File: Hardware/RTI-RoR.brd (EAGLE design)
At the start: 80 x 71.1 mm, 49 parts, among them IC1 24AA128ST, IC3 FT232RL, IC5 74LVC245, IC6 74ABT245, X13 PN61729-S

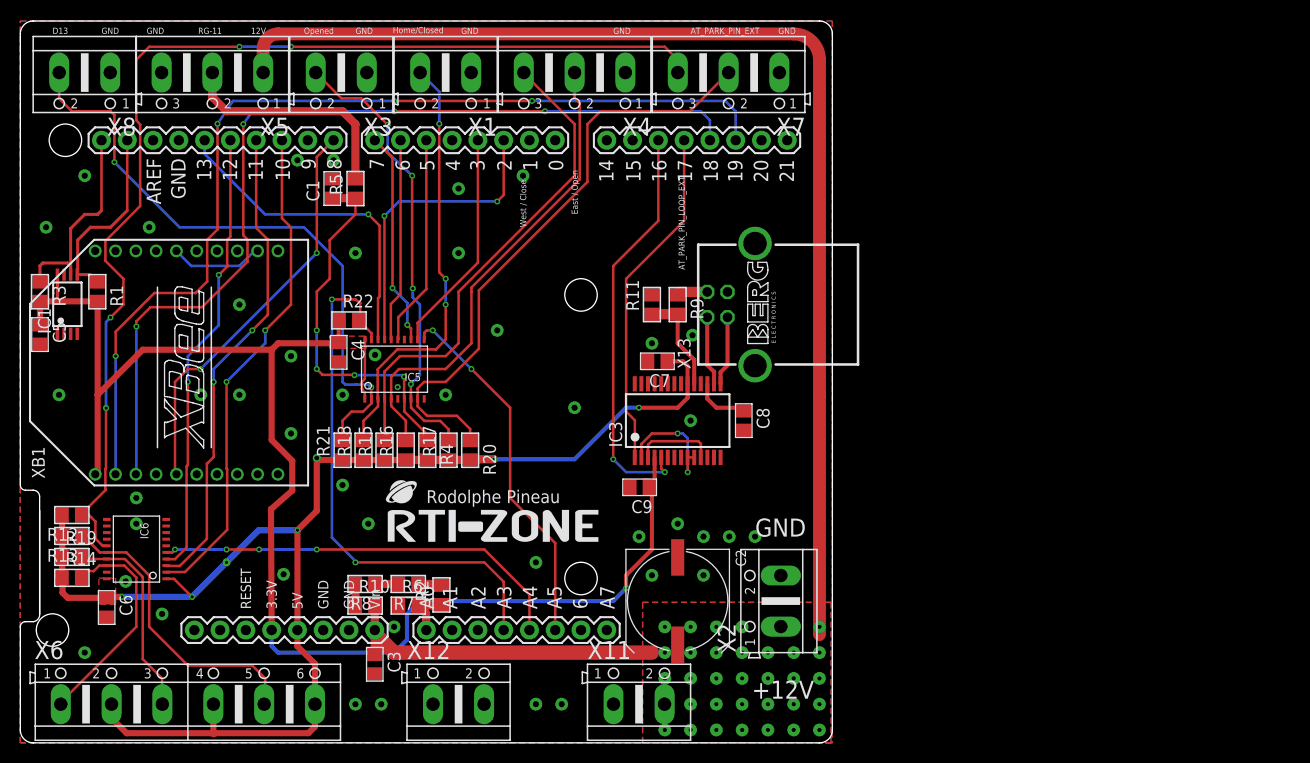
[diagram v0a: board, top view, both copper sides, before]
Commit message: Re-base the code with the dome code
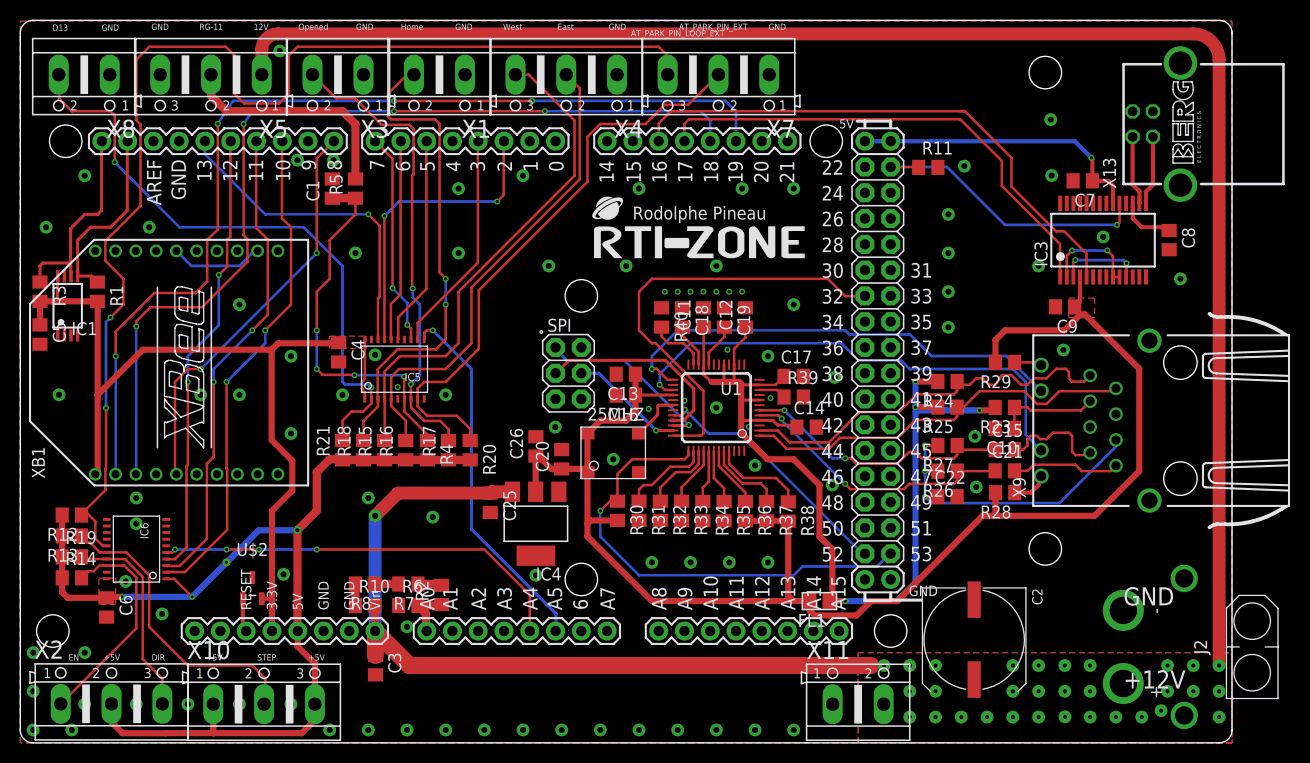
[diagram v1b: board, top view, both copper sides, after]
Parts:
- removed PCB1: ARDUINO_DUE_SHIELD_SHORT, arduino_shield:ARDUINO_DUE_SHIELD_SHORT
- removed R22, R9: 4.7K, rti:R0805
- removed X12: (no value), con-ptr500:AK500/2
- removed X6: (no value), con-ptr500:AK500/6
- added 25MHZ: CB3LV-OSCILATOR, rti:SMD-7050_4P
- added C10: 22nF, rcl:C0805
- added C11, C12, C14, C16, C17, C20: 100nF, rcl:C0805
- added C13, C18, C22: 10nF, rcl:C0805
- added C15, C21: 6.8nF, rcl:C0805
- added C19: 4.7uF, rcl:C0805
- added C25, C26: 10uF, rcl:C0805
- added FL1: BLM21AG121SN1D, BLM21AG121SN1D:L0805
- added IC4: REG1117, burr-brown:SOT223
- added J2: XT60PW-M, samacsys:XT60PWM
- added R23: 10 1%, rcl:R0805
- added R24, R25, R26, R27: 49.9 1%, rcl:R0805
- added R28, R29: 330, rcl:R0805
- added R30, R31, R32, R33, R34, R35, R36, R37, R38, R40: 4.7K, rcl:R0805
- added R39: 12.4K 1%, rcl:R0805
- added U$1: ARDUINO_DUE_SHIELD_FULL, arduino_shield:ARDUINO_DUE_SHIELD_FULL
- added U$2: MCP120T-270I_TT, MCP120T-270I_TT:SOT95P237X112-3N
- added U1: W5500, W5500:LQFP48
- added X10: (no value), rti:AK500/3
- added X9: J1011F21PNL, rti:J1011F21PNL
- C1, C3, C4, C5, C6, C7, C8, C9: device rti:C0805 -> rcl:C0805
- C2: device rti:UD-10X10_NICHICON -> rcl:UD-10X10_NICHICON
- IC1: device microchip:TSSOP8 -> rti:TSSOP8
- R1, R10, R11, R12, R13, R14, R15, R16, R17, R18, R19, R2, R20, R21, R3, R4, R5, R6, R7, R8: device rti:R0805 -> rcl:R0805
- X1, X11, X3, X8: device con-ptr500:AK500/2 -> rti:AK500/2
- X13: device con-berg:PN61729-S -> rti:PN61729-S
- X2: device con-ptr500:AK500/2 -> rti:AK500/3
- X4, X5, X7: device con-ptr500:AK500/3 -> rti:AK500/3
- XB1: device maxstream:XBEE -> rti:XBEE
- moved X2 66.7 mm to (8.99, 3.84), turned to 0 degrees
- moved IC3 45.5 mm to (106.7, 49.5)
- moved C7 45.5 mm to (104.7, 55.4)
- moved C8 45.5 mm to (113.2, 49.5)
- moved C9 45.5 mm to (102.9, 43.0)
- moved X13 45.5 mm to (114.3, 61.0)
- moved U$4 34.5 mm to (56.5, 47.8)
- moved R11 30.4 mm to (89.5, 56.7), turned to 0 degrees
- moved C2 29.5 mm to (94.0, 10.2)
- moved X11 21.6 mm to (82.5, 3.81)
- moved X7 1.02 mm to (68.8, 65.8)
- moved X4 0.85 mm to (53.8, 65.8)
- moved X1 0.64 mm to (41.3, 65.8)
- moved X3 0.38 mm to (31.3, 65.8)
- moved X5 0.24 mm to (18.8, 65.8)
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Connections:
- removed net BUF_EN: IC5.P$19, PCB1.A3, R22.2
- removed net N$1: IC3.19, R11.1, R9.2
- new net +3V3: 25MHZ.1, 25MHZ.4, C13.1, C16.1, C20.1, C26.1, C9.1, FL1.2, IC3.4, IC4.2, R28.2, R29.2, R30.2, R36.2, R37.2, R38.2, U1.28
- new net +5V: U$1.+5V@2
- new net ACT_LED: U1.27, X9.11
- new net AVDD: C11.1, C12.1, C14.1, C17.1, FL1.1, R23.2, R24.2, R25.2, U1.11, U1.15, U1.17, U1.21, U1.4, U1.8
- new net ETH_CS: U$1.52, U1.32
- new net ETH_RESET: R30.1, U$1.53, U1.37
- new net FTDI_RESET: IC3.19, R11.1, U$1.23
- new net INT_N: U$1.32, U1.36
- new net LINK_ACK: U1.25, X9.10
- new net N$10: R28.1, X9.12
- new net N$11: C15.2, X9.7
- new net N$12: C21.2, X9.8
- new net N$13: C10.1, R23.1, X9.3
- new net N$17: U1.26
- new net N$22: R31.1, U1.38
- new net N$23: R32.1, U1.39
- new net N$24: R33.1, U1.40
- new net N$25: R34.1, U1.41
- new net N$26: R35.1, U1.42
- new net N$27: R36.1, U1.43
- new net N$28: R37.1, U1.44
- new net N$29: R38.1, U1.45
- new net N$31: C19.2, U1.20
- new net N$32: U1.18
- new net N$33: C18.2, U1.22
- new net N$34: R39.1, U1.10
- new net N$35: R40.2, U1.23
- new net N$7: C22.1, R26.2, R27.2, X9.6
- new net N$8: R29.1, X9.9
- new net RESET: U$1.RESET, U$2.1
- new net RXN: C21.1, R26.1, U1.5
- new net RXP: C15.1, R27.1, U1.6
- new net SCLK: U$1.SCK, U1.33
- new net SDI: U$1.MISO, U1.34
- new net SDO: U$1.MOSI, U1.35
- new net TXN: R25.1, U1.1, X9.2
- new net TXP: R24.1, U1.2, X9.1
- new net XI: 25MHZ.3, U1.30
- new net XO: U1.31
- net +12V: now also C25.1, IC4.3, J2.2, U$1.VIN; no longer PCB1.VIN, X2.1
- net 3.3V: now also U$1.3.3V, U$2.2; no longer C9.1, IC3.4, PCB1.3.3V, R22.1
- net AT_PARK_PIN: now also U$1.A5; no longer PCB1.A5
- net AT_PARK_PIN_LOOP: now also U$1.A4; no longer PCB1.A4
- net BUTTON_EAST_OPEN: now also U$1.5; no longer PCB1.5
- net BUTTON_WEST_CLOSE: now also U$1.6; no longer PCB1.6
- net D13: now also U$1.13; no longer PCB1.13
- net GND: now also 25MHZ.2, C10.2, C11.2, C12.2, C13.2, C14.2, C16.2, C17.2, C18.1, C19.1, C20.2, C22.2, C25.2, C26.2, IC4.1, IC5.P$19, J2.1, R31.2, R32.2, R33.2, R34.2, R35.2, R39.2, R40.1, U$1.GND, U$1.GND., U$1.GND.., U$1.GND..., U$1.GND...., U$1.GND__, U$2.3, U1.14, U1.16, U1.19, U1.29, U1.3, U1.48, U1.9, X9.4, X9.5, X9.M1, X9.M2; no longer PCB1.GND, PCB1.GND., PCB1.GND.., X12.1, X12.2, X2.2
- net HOME_SHUTTER_CLOSED: now also U$1.2; no longer PCB1.2
- net M_DIR: now also U$1.11; no longer PCB1.11
- net M_DIR_5V: now also X2.3; no longer X6.3
- net M_EN: now also U$1.10; no longer PCB1.10
- net M_EN_5V: now also X2.1; no longer X6.1
- net M_STEP: now also U$1.12; no longer PCB1.12
- net M_STEP_5V: now also X10.2; no longer X6.5
- net RG-11: now also U$1.7; no longer PCB1.7
- net RX2: now also U$1.17; no longer PCB1.17
- net SCL: now also U$1.SCL1; no longer PCB1.SCL1
- net SDA: now also U$1.SDA1; no longer PCB1.SDA1
- net SHUTTER_OPENED: now also U$1.3; no longer PCB1.3
- net TX2: now also U$1.16; no longer PCB1.16
- net USB_VCC: no longer R9.1
- net VCC: now also U$1.+5V@1, U$1.+5V@3, U$1.+5V@4, X10.1, X10.3, X2.2; no longer PCB1.5V, X6.2, X6.4, X6.6
- net VPIN: now also U$1.A0; no longer PCB1.A0
- net XBEE_DIN: now also U$1.18; no longer PCB1.18
- net XBEE_DOUT: now also U$1.19; no longer PCB1.19
- net XBEE_RESET: now also U$1.8; no longer PCB1.8
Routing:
- net +3V3: track 0.00 -> 146.7 mm
- net AVDD: track 0.00 -> 96.8 mm, vias 0 -> 4
- net +12V: track 148.7 -> 239.2 mm
- net 3.3V: track 146.4 -> 90.1 mm, vias 1 -> 0
- net BUF_EN: track 54.1 -> 0.00 mm, vias 2 -> 0
- net ACT_LED: track 0.00 -> 48.9 mm, vias 0 -> 1
- net ETH_RESET: track 0.00 -> 46.6 mm, vias 0 -> 1
- net LINK_ACK: track 0.00 -> 45.7 mm, vias 0 -> 1
- net INT_N: track 0.00 -> 43.4 mm
- net TXN: track 0.00 -> 39.7 mm
- net TXP: track 0.00 -> 39.4 mm
- net N$7: track 0.00 -> 30.8 mm, vias 0 -> 3
- net FTDI_RESET: track 0.00 -> 29.7 mm, vias 0 -> 1
- net RXN: track 0.00 -> 27.6 mm, vias 0 -> 2
- net RXP: track 0.00 -> 27.4 mm, vias 0 -> 2
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- added copper zone on layer 1, net +3V3
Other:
- board size 80 x 71.1 mm -> 119.4 x 71.2 mm
- board text added: "+5V"
- board text added: "DIR"
- board text added: "Dome Rotator"
- board text added: "EN"
- board text added: "East"
- board text added: "Home"
- board text added: "STEP"
- board text added: "West"
- board text removed: "East / Open"
- board text removed: "Home/Closed"
- board text removed: "West / Close"
